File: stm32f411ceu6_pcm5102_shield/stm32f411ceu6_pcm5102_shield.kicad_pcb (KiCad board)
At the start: 4 copper layers, 74 parts, among them J100 Conn_01x04_Pin, J101 Conn_01x04_Pin, J102 Conn_01x04_Pin, J200 AudioJack3_Ground_SwitchTR, J201 Conn_01x03_Pin, J300 AudioJack3_Ground_SwitchTR, J301 Conn_01x03_Pin, Q300 BC337, Q301 BC337, SW100 RotaryEncoder_Switch_MP, SW200 SW_DPDT_XLX, U100 BlackPill, U101 INMP411, U200 PCM5102A, U201 HT7533-1

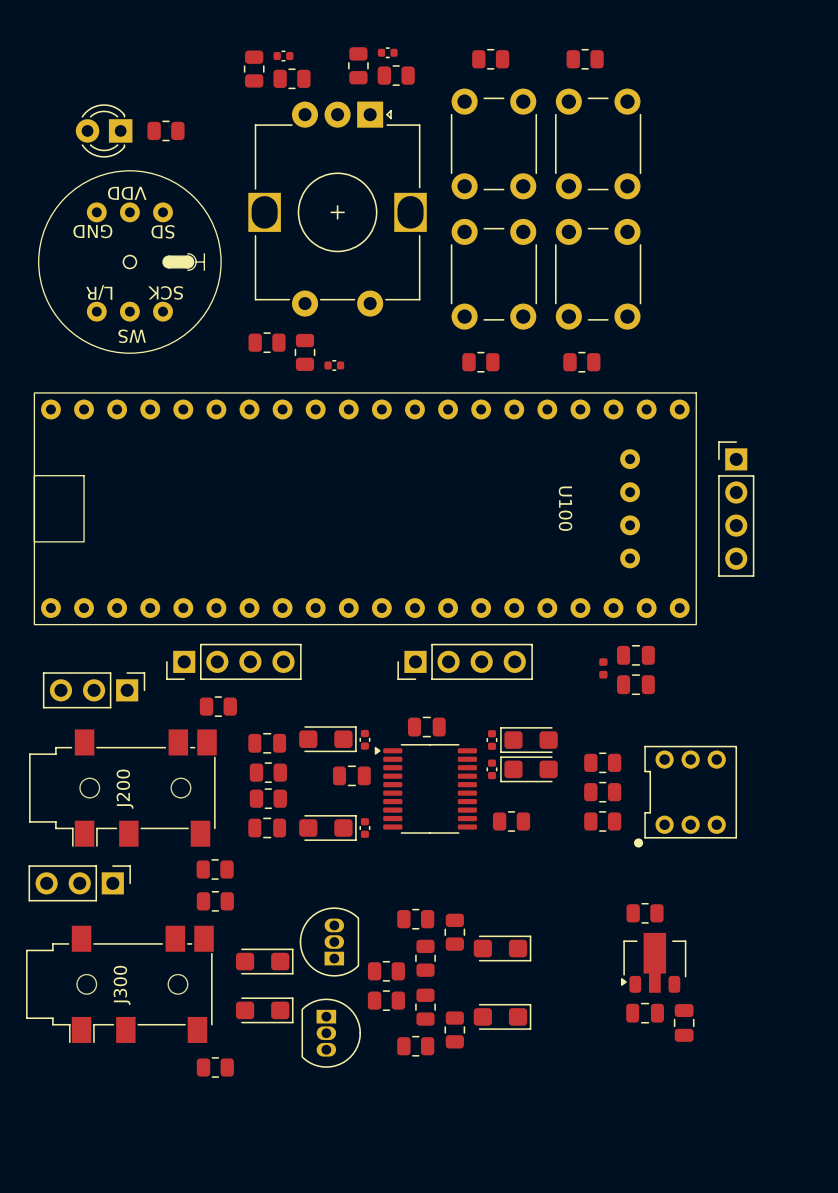
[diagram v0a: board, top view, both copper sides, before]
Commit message: Board outline
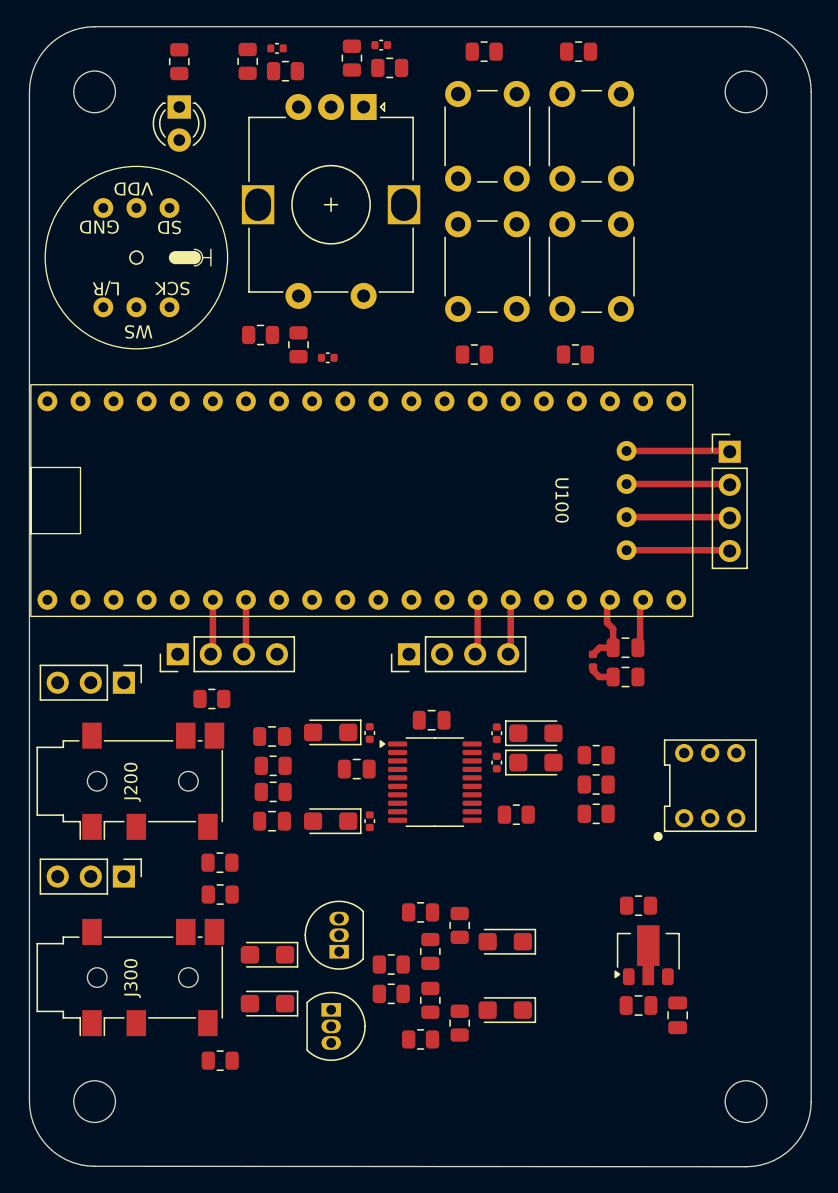
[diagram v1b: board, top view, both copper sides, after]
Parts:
- added H1: MountingHole, MountingHole:MountingHole_3.2mm_M3, F.Cu at (80.2, 55.0)
- added H2: MountingHole, MountingHole:MountingHole_3.2mm_M3, F.Cu at (130.2, 55.0)
- added H3: MountingHole, MountingHole:MountingHole_3.2mm_M3, F.Cu at (130.2, 132.5)
- added H4: MountingHole, MountingHole:MountingHole_3.2mm_M3, F.Cu at (80.2, 132.5)
- moved R110 5.41 mm to (86.8, 52.7), turned to 90 degrees
- moved D1 4.86 mm to (86.8, 56.2), turned to -90 degrees
- moved SW200 1.58 mm to (127.5, 108.2)
- moved J301 1.00 mm to (82.5, 115.2)
- moved C200 0.99 mm to (121.0, 97.7)
- moved C201 0.99 mm to (121.0, 99.9)
- moved L200 0.99 mm to (118.5, 98.7)
- moved J300 0.96 mm to (79.8, 123.0)
- moved J200 0.77 mm to (79.8, 107.9)
- moved C100 0.77 mm to (98.2, 75.4)
- moved C202 0.77 mm to (122.0, 125.1)
- moved C203 0.77 mm to (125.0, 125.9)
- moved J101 0.77 mm to (86.6, 98.2)
- moved J102 0.77 mm to (104.4, 98.2)
- moved R100 0.77 mm to (95.9, 74.4)
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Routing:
- net Net-(J100-Pin_4): track 0.00 -> 7.95 mm
- net Net-(J100-Pin_3): track 0.00 -> 7.95 mm
- net Net-(J100-Pin_2): track 0.00 -> 7.95 mm
- net Net-(J100-Pin_1): track 0.00 -> 7.95 mm
- net +5V: track 0.00 -> 5.59 mm
- net /MCU/I2C1_SCL: track 0.00 -> 4.25 mm
- net /MCU/I2C1_SDA: track 0.00 -> 4.25 mm
- net /MCU/USART1_RX: track 0.00 -> 4.24 mm
- net /MCU/USART1_TX: track 0.00 -> 4.24 mm
- net GND: track 0.00 -> 3.70 mm
- net +5VA: track 0.00 -> 2.02 mm
- added copper zone on In1.Cu, net GND
- added copper zone on In2.Cu, net GND
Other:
- board outline added: 60 x 87.5 mm
